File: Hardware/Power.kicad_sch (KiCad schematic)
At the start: 28 parts, among them U2 TPS54302, U3 LD1086DT33TR, U8 TPS2121RUXR

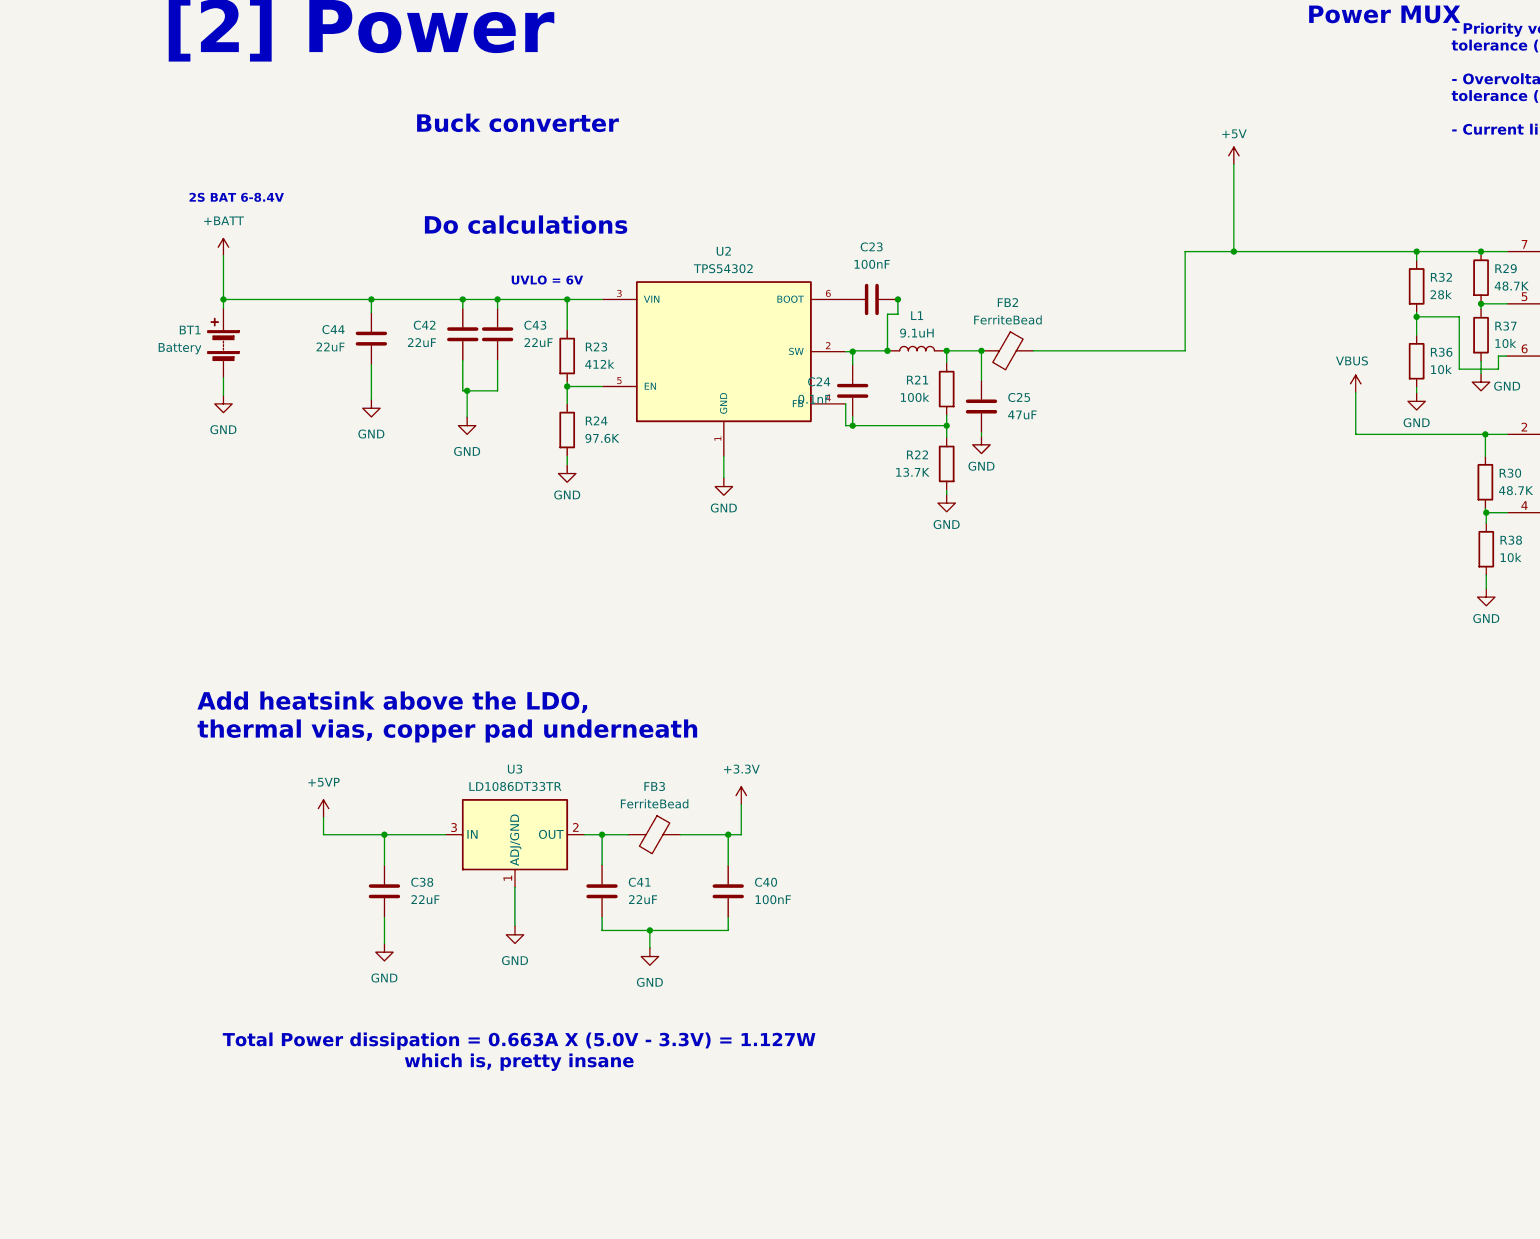
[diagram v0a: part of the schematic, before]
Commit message: Commit bulamadim :)
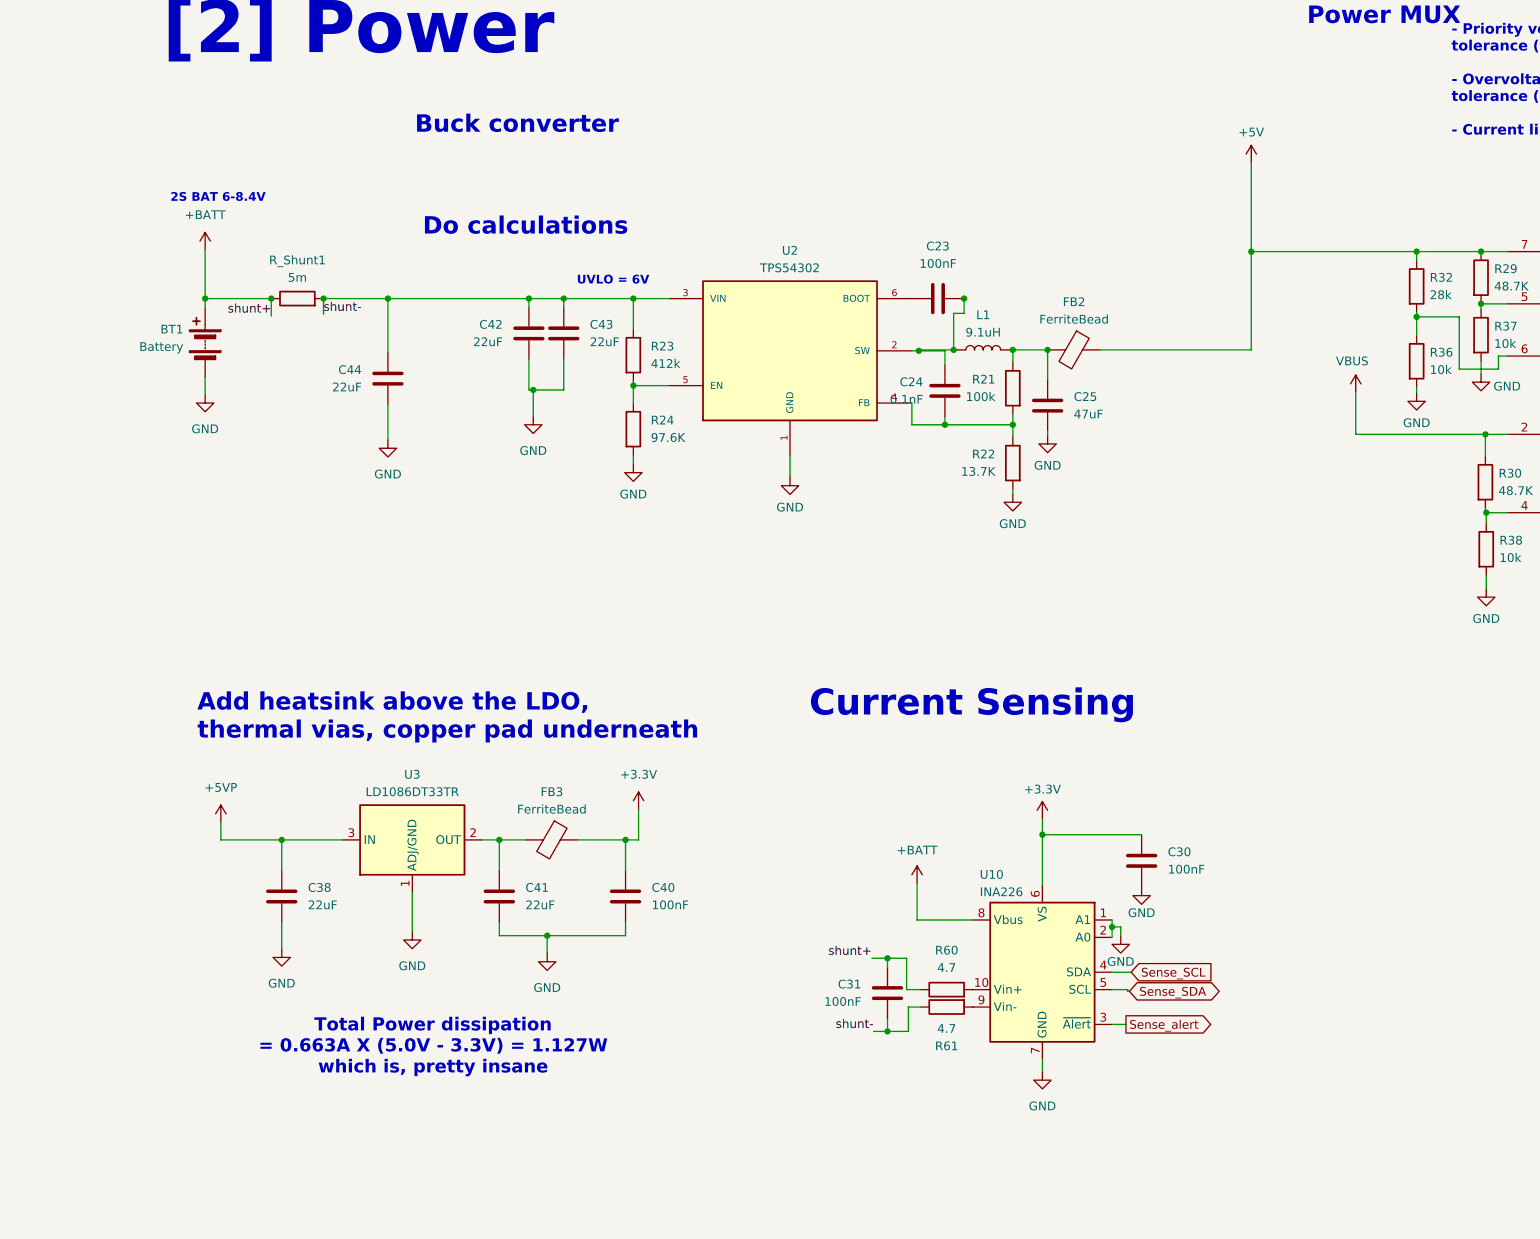
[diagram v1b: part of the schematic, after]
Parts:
- added C30, C31: 100nF, Capacitor_SMD:C_0402_1005Metric, symbol Device:C
- added R60, R61: 4.7, Resistor_SMD:R_0402_1005Metric, symbol Device:R
- added R_Shunt1: 5m, Resistor_SMD:R_1206_3216Metric, symbol Device:R
- added U10: INA226, Package_SO:TSSOP-10_3x3mm_P0.5mm, symbol Sensor_Energy:INA226
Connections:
- net +3.3V: now also C30.1, U10.6 (VS)
- net +BATT: now also C31.1, R60.1, R_Shunt1.1, U10.8 (Vbus); no longer C42.1, C43.1, C44.1, R23.1, U2.3 (VIN)
- net GND: now also C30.2, U10.1 (A1), U10.2 (A0), U10.7 (GND)
- new net: R60.2, U10.10 (Vin+)
- new net: R61.2, U10.9 (Vin-)
- new net: C42.1, C43.1, R23.1, U2.3 (VIN)
- new net Sense_SCL: U10.4 (SDA)
- new net Sense_SDA: U10.5 (SCL)
- new net Sense_alert: U10.3 (~{Alert})
- new net shunt-: C31.2, C44.1, R61.1, R_Shunt1.2
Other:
- note added: "Current Sensing"
- moved on the sheet: BT1, C23, C24, C25, C38, C40, C41, C42, C43, C44, FB2, FB3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
